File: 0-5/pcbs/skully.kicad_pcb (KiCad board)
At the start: 2 copper layers, 125.9 x 109.4 mm, 1 part

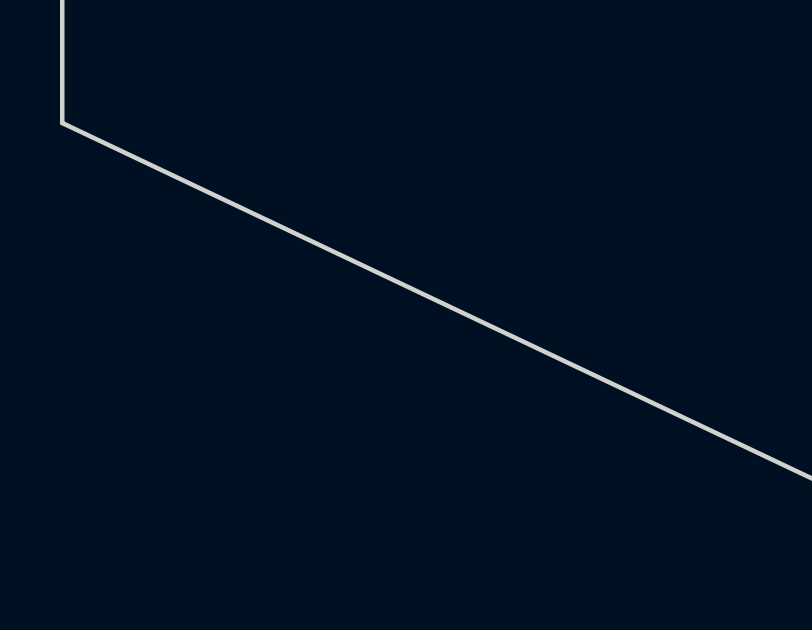
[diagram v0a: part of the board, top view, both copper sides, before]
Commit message: keys footprint working somehow
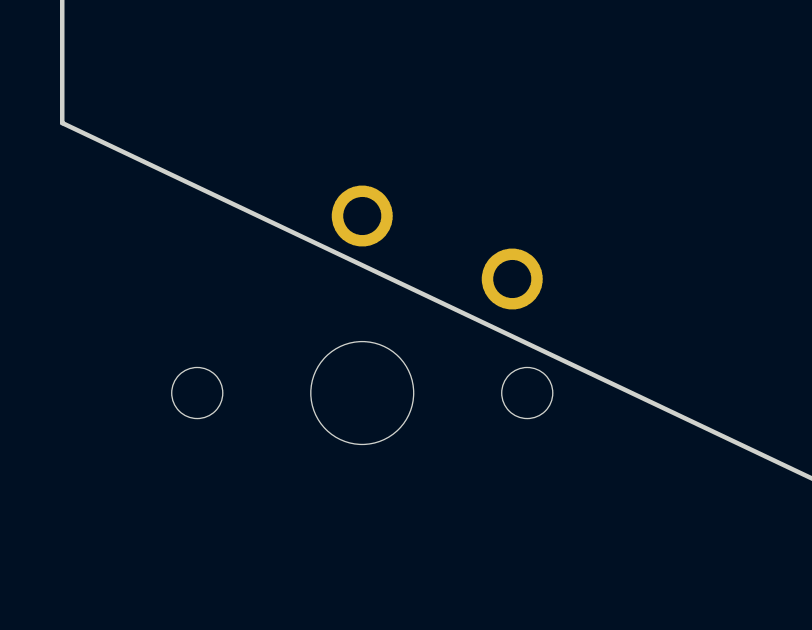
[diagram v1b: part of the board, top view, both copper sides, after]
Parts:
- added S1: , PG1350, F.Cu at (0.00, 0.00)
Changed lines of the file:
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@@
   )
             (net 0 "")
-(net 1 "RAW")
-(net 2 "GND")
-(net 3 "RST")
-(net 4 "VCC")
-(net 5 "P21")
-(net 6 "P20")
-(net 7 "P19")
-(net 8 "P18")
-(net 9 "P15")
-(net 10 "P14")
-(net 11 "P16")
-(net 12 "P10")
-(net 13 "P1")
-(net 14 "P0")
-(net 15 "P2")
-(net 16 "P3")
-(net 17 "P4")
-(net 18 "P5")
-(net 19 "P6")
-(net 20 "P7")
-(net 21 "P8")
-(net 22 "P9")
+(net 1 "=column_net")
+(net 2 "RAW")
+(net 3 "GND")
+(net 4 "RST")
+(net 5 "VCC")
+(net 6 "P21")
+(net 7 "P20")
+(net 8 "P19")
+(net 9 "P18")
+(net 10 "P15")
+(net 11 "P14")
+(net 12 "P16")
+(net 13 "P10")
+(net 14 "P1")
+(net 15 "P0")
+(net 16 "P2")
+(net 17 "P3")
+(net 18 "P4")
+(net 19 "P5")
+(net 20 "P6")
+(net 21 "P7")
+(net 22 "P8")
+(net 23 "P9")
   (net_class Default "This is the default net class."
     (clearance 0.2)
@@
     (uvia_drill 0.1)
     (add_net "")
+(add_net "=column_net")
 (add_net "RAW")
 (add_net "GND")
@@
 (add_net "P9")
   )
+      (module PG1350 (layer F.Cu)
+      (at 0 0 0)
+      (fp_text reference "S1" (at 0 0) (layer F.SilkS) hide (effects (font (size 1.27 1.27) (thickness 0.15))))
+      (fp_text value "" (at 0 0) (layer F.SilkS) hide (effects (font (size 1.27 1.27) (thickness 0.15))))
+      (fp_line (start -7 -6) (end -7 -7) (layer Dwgs.User) (width 0.15))
+      (fp_line (start -7 7) (end -6 7) (layer Dwgs.User) (width 0.15))
+      (fp_line (start -6 -7) (end -7 -7) (layer Dwgs.User) (width 0.15))
+      (fp_line (start -7 7) (end -7 6) (layer Dwgs.User) (width 0.15))
+      (fp_line (start 7 6) (end 7 7) (layer Dwgs.User) (width 0.15))
+      (fp_line (start 7 -7) (end 6 -7) (layer Dwgs.User) (width 0.15))
+      (fp_line (start 6 7) (end 7 7) (layer Dwgs.User) (width 0.15))
+      (fp_line (start 7 -7) (end 7 -6) (layer Dwgs.User) (width 0.15))
+      (pad "" np_thru_hole circle (at 0 0) (size 3.429 3.429) (drill 3.429) (layers *.Cu *.Mask))
+      (pad "" np_thru_hole circle (at 5.5 0) (size 1.7018 1.7018) (drill 1.7018) (layers *.Cu *.Mask))
+      (pad "" np_thru_hole circle (at -5.5 0) (size 1.7018 1.7018) (drill 1.7018) (layers *.Cu *.Mask))
+      (fp_line (start -9 -8.5) (end 9 -8.5) (layer Dwgs.User) (width 0.15))
+      (fp_line (start 9 -8.5) (end 9 8.5) (layer Dwgs.User) (width 0.15))
+      (fp_line (start 9 8.5) (end -9 8.5) (layer Dwgs.User) (width 0.15))
+      (fp_line (start -9 8.5) (end -9 -8.5) (layer Dwgs.User) (width 0.15))
+            (pad 1 thru_hole circle (at 5 -3.8) (size 2.032 2.032) (drill 1.27) (layers *.Cu *.Mask) (net 1 "=column_net"))
+            (pad 2 thru_hole circle (at 0 -5.9) (size 2.032 2.032) (drill 1.27) (layers *.Cu *.Mask) (net 1 "=column_net"))
+          )
       (module ProMicro (layer F.Cu)
       (at 103.2380534 -25.506203899999996 -98.6)
@@
         (fp_text user P08 (at 11.43 -4.8 -8.599999999999994) (layer F.SilkS) (effects (font (size 0.8 0.8) (thickness 0.15))))
         (fp_text user P09 (at 13.97 -4.8 -8.599999999999994) (layer F.SilkS) (effects (font (size 0.8 0.8) (thickness 0.15))))
-        (pad 1 thru_hole rect (at -13.97 7.62 -98.6) (size 1.7526 1.7526) (drill 1.0922) (layers *.Cu *.SilkS *.Mask) (net 1 "RAW"))
-        (pad 2 thru_hole circle (at -11.43 7.62 0) (size 1.7526 1.7526) (drill 1.0922) (layers *.Cu *.SilkS *.Mask) (net 2 "GND"))
-        (pad 3 thru_hole circle (at -8.89 7.62 0) (size 1.7526 1.7526) (drill 1.0922) (layers *.Cu *.SilkS *.Mask) (net 3 "RST"))
-        (pad 4 thru_hole circle (at -6.35 7.62 0) (size 1.7526 1.7526) (drill 1.0922) (layers *.Cu *.SilkS *.Mask) (net 4 "VCC"))
-        (pad 5 thru_hole circle (at -3.81 7.62 0) (size 1.7526 1.7526) (drill 1.0922) (layers *.Cu *.SilkS *.Mask) (net 5 "P21"))
-        (pad 6 thru_hole circle (at -1.27 7.62 0) (size 1.7526 1.7526) (drill 1.0922) (layers *.Cu *.SilkS *.Mask) (net 6 "P20"))
-        (pad 7 thru_hole circle (at 1.27 7.62 0) (size 1.7526 1.7526) (drill 1.0922) (layers *.Cu *.SilkS *.Mask) (net 7 "P19"))
-        (pad 8 thru_hole circle (at 3.81 7.62 0) (size 1.7526 1.7526) (drill 1.0922) (layers *.Cu *.SilkS *.Mask) (net 8 "P18"))
-        (pad 9 thru_hole circle (at 6.35 7.62 0) (size 1.7526 1.7526) (drill 1.0922) (layers *.Cu *.SilkS *.Mask) (net 9 "P15"))
-        (pad 10 thru_hole circle (at 8.89 7.62 0) (size 1.7526 1.7526) (drill 1.0922) (layers *.Cu *.SilkS *.Mask) (net 10 "P14"))
-        (pad 11 thru_hole circle (at 11.43 7.62 0) (size 1.7526 1.7526) (drill 1.0922) (layers *.Cu *.SilkS *.Mask) (net 11 "P16"))
-        (pad 12 thru_hole circle (at 13.97 7.62 0) (size 1.7526 1.7526) (drill 1.0922) (layers *.Cu *.SilkS *.Mask) (net 12 "P10"))
-        (pad 13 thru_hole circle (at -13.97 -7.62 0) (size 1.7526 1.7526) (drill 1.0922) (layers *.Cu *.SilkS *.Mask) (net 13 "P1"))
-        (pad 14 thru_hole circle (at -11.43 -7.62 0) (size 1.7526 1.7526) (drill 1.0922) (layers *.Cu *.SilkS *.Mask) (net 14 "P0"))
-        (pad 15 thru_hole circle (at -8.89 -7.62 0) (size 1.7526 1.7526) (drill 1.0922) (layers *.Cu *.SilkS *.Mask) (net 2 "GND"))
-        (pad 16 thru_hole circle (at -6.35 -7.62 0) (size 1.7526 1.7526) (drill 1.0922) (layers *.Cu *.SilkS *.Mask) (net 2 "GND"))
-        (pad 17 thru_hole circle (at -3.81 -7.62 0) (size 1.7526 1.7526) (drill 1.0922) (layers *.Cu *.SilkS *.Mask) (net 15 "P2"))
-        (pad 18 thru_hole circle (at -1.27 -7.62 0) (size 1.7526 1.7526) (drill 1.0922) (layers *.Cu *.SilkS *.Mask) (net 16 "P3"))
-        (pad 19 thru_hole circle (at 1.27 -7.62 0) (size 1.7526 1.7526) (drill 1.0922) (layers *.Cu *.SilkS *.Mask) (net 17 "P4"))
-        (pad 20 thru_hole circle (at 3.81 -7.62 0) (size 1.7526 1.7526) (drill 1.0922) (layers *.Cu *.SilkS *.Mask) (net 18 "P5"))
-        (pad 21 thru_hole circle (at 6.35 -7.62 0) (size 1.7526 1.7526) (drill 1.0922) (layers *.Cu *.SilkS *.Mask) (net 19 "P6"))
-        (pad 22 thru_hole circle (at 8.89 -7.62 0) (size 1.7526 1.7526) (drill 1.0922) (layers *.Cu *.SilkS *.Mask) (net 20 "P7"))
-        (pad 23 thru_hole circle (at 11.43 -7.62 0) (size 1.7526 1.7526) (drill 1.0922) (layers *.Cu *.SilkS *.Mask) (net 21 "P8"))
-        (pad 24 thru_hole circle (at 13.97 -7.62 0) (size 1.7526 1.7526) (drill 1.0922) (layers *.Cu *.SilkS *.Mask) (net 22 "P9"))
+        (pad 1 thru_hole rect (at -13.97 7.62 -98.6) (size 1.7526 1.7526) (drill 1.0922) (layers *.Cu *.SilkS *.Mask) (net 2 "RAW"))
+        (pad 2 thru_hole circle (at -11.43 7.62 0) (size 1.7526 1.7526) (drill 1.0922) (layers *.Cu *.SilkS *.Mask) (net 3 "GND"))
+        (pad 3 thru_hole circle (at -8.89 7.62 0) (size 1.7526 1.7526) (drill 1.0922) (layers *.Cu *.SilkS *.Mask) (net 4 "RST"))
+        (pad 4 thru_hole circle (at -6.35 7.62 0) (size 1.7526 1.7526) (drill 1.0922) (layers *.Cu *.SilkS *.Mask) (net 5 "VCC"))
+        (pad 5 thru_hole circle (at -3.81 7.62 0) (size 1.7526 1.7526) (drill 1.0922) (layers *.Cu *.SilkS *.Mask) (net 6 "P21"))
+        (pad 6 thru_hole circle (at -1.27 7.62 0) (size 1.7526 1.7526) (drill 1.0922) (layers *.Cu *.SilkS *.Mask) (net 7 "P20"))
+        (pad 7 thru_hole circle (at 1.27 7.62 0) (size 1.7526 1.7526) (drill 1.0922) (layers *.Cu *.SilkS *.Mask) (net 8 "P19"))
+        (pad 8 thru_hole circle (at 3.81 7.62 0) (size 1.7526 1.7526) (drill 1.0922) (layers *.Cu *.SilkS *.Mask) (net 9 "P18"))
+        (pad 9 thru_hole circle (at 6.35 7.62 0) (size 1.7526 1.7526) (drill 1.0922) (layers *.Cu *.SilkS *.Mask) (net 10 "P15"))
+        (pad 10 thru_hole circle (at 8.89 7.62 0) (size 1.7526 1.7526) (drill 1.0922) (layers *.Cu *.SilkS *.Mask) (net 11 "P14"))
+        (pad 11 thru_hole circle (at 11.43 7.62 0) (size 1.7526 1.7526) (drill 1.0922) (layers *.Cu *.SilkS *.Mask) (net 12 "P16"))
+        (pad 12 thru_hole circle (at 13.97 7.62 0) (size 1.7526 1.7526) (drill 1.0922) (layers *.Cu *.SilkS *.Mask) (net 13 "P10"))
+        (pad 13 thru_hole circle (at -13.97 -7.62 0) (size 1.7526 1.7526) (drill 1.0922) (layers *.Cu *.SilkS *.Mask) (net 14 "P1"))
+        (pad 14 thru_hole circle (at -11.43 -7.62 0) (size 1.7526 1.7526) (drill 1.0922) (layers *.Cu *.SilkS *.Mask) (net 15 "P0"))
+        (pad 15 thru_hole circle (at -8.89 -7.62 0) (size 1.7526 1.7526) (drill 1.0922) (layers *.Cu *.SilkS *.Mask) (net 3 "GND"))
+        (pad 16 thru_hole circle (at -6.35 -7.62 0) (size 1.7526 1.7526) (drill 1.0922) (layers *.Cu *.SilkS *.Mask) (net 3 "GND"))
+        (pad 17 thru_hole circle (at -3.81 -7.62 0) (size 1.7526 1.7526) (drill 1.0922) (layers *.Cu *.SilkS *.Mask) (net 16 "P2"))
+        (pad 18 thru_hole circle (at -1.27 -7.62 0) (size 1.7526 1.7526) (drill 1.0922) (layers *.Cu *.SilkS *.Mask) (net 17 "P3"))
+        (pad 19 thru_hole circle (at 1.27 -7.62 0) (size 1.7526 1.7526) (drill 1.0922) (layers *.Cu *.SilkS *.Mask) (net 18 "P4"))
+        (pad 20 thru_hole circle (at 3.81 -7.62 0) (size 1.7526 1.7526) (drill 1.0922) (layers *.Cu *.SilkS *.Mask) (net 19 "P5"))
+        (pad 21 thru_hole circle (at 6.35 -7.62 0) (size 1.7526 1.7526) (drill 1.0922) (layers *.Cu *.SilkS *.Mask) (net 20 "P6"))
+        (pad 22 thru_hole circle (at 8.89 -7.62 0) (size 1.7526 1.7526) (drill 1.0922) (layers *.Cu *.SilkS *.Mask) (net 21 "P7"))
+        (pad 23 thru_hole circle (at 11.43 -7.62 0) (size 1.7526 1.7526) (drill 1.0922) (layers *.Cu *.SilkS *.Mask) (net 22 "P8"))
+        (pad 24 thru_hole circle (at 13.97 -7.62 0) (size 1.7526 1.7526) (drill 1.0922) (layers *.Cu *.SilkS *.Mask) (net 23 "P9"))
       )
             (gr_line (start 107.54047 14.161463800000003) (end 115.9067447 -42.5943362) (angle 90) (layer Edge.Cuts) (width 0.15))
